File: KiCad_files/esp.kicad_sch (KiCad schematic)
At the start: 0 parts

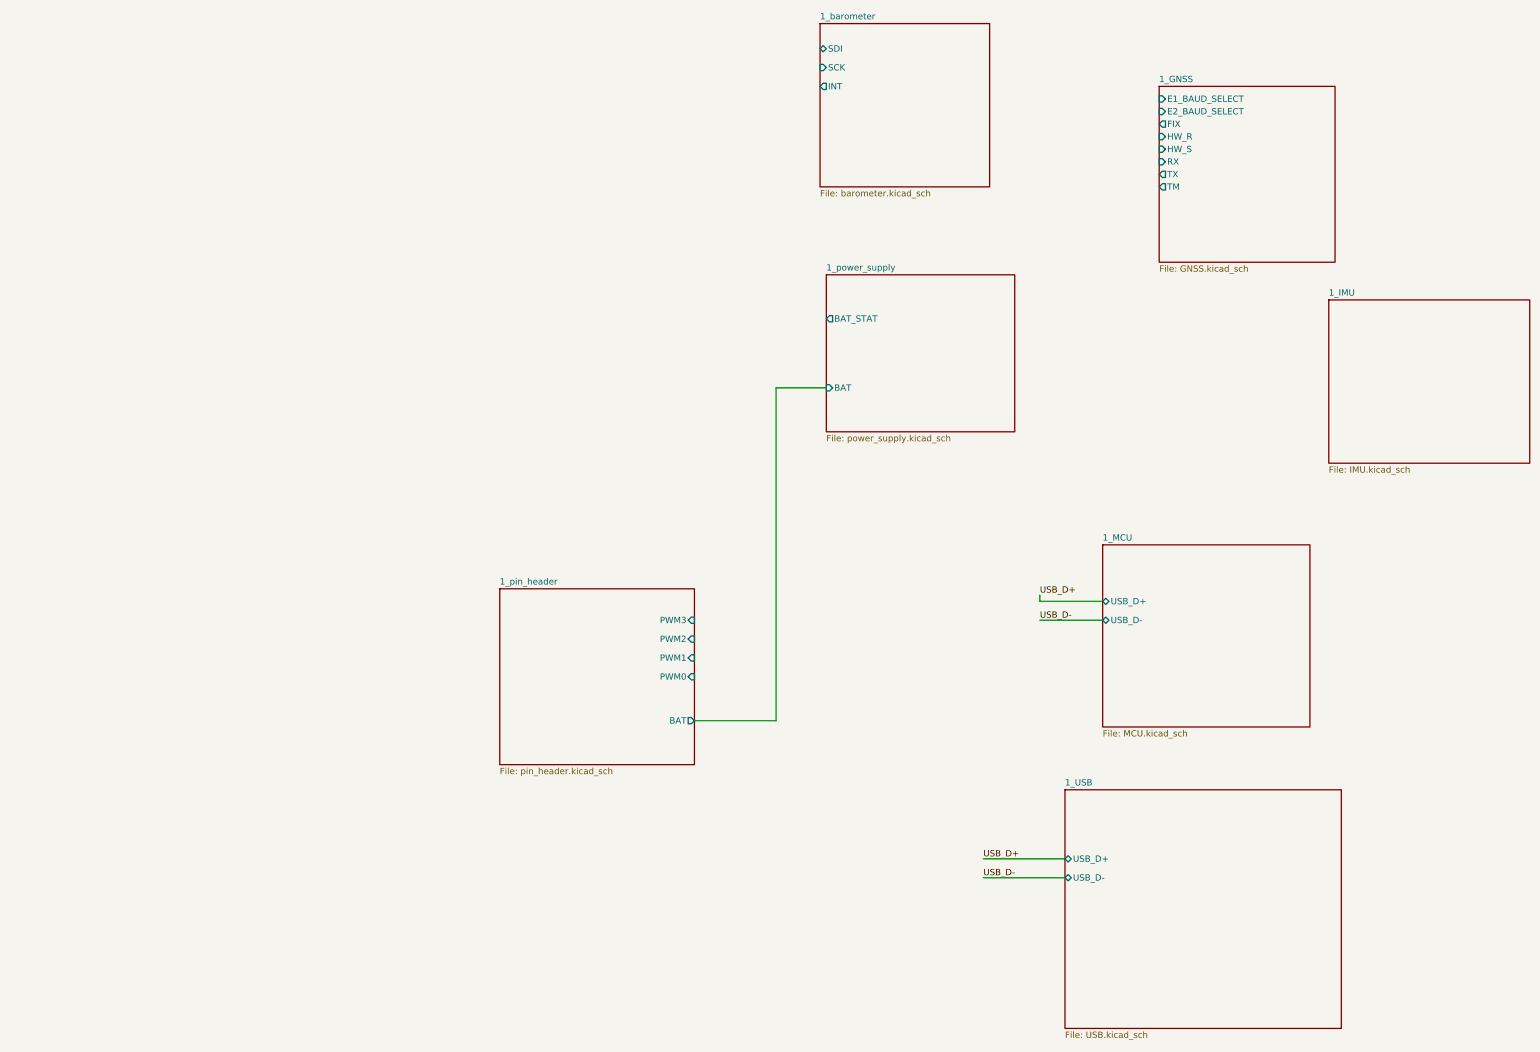
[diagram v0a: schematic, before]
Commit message: i2c
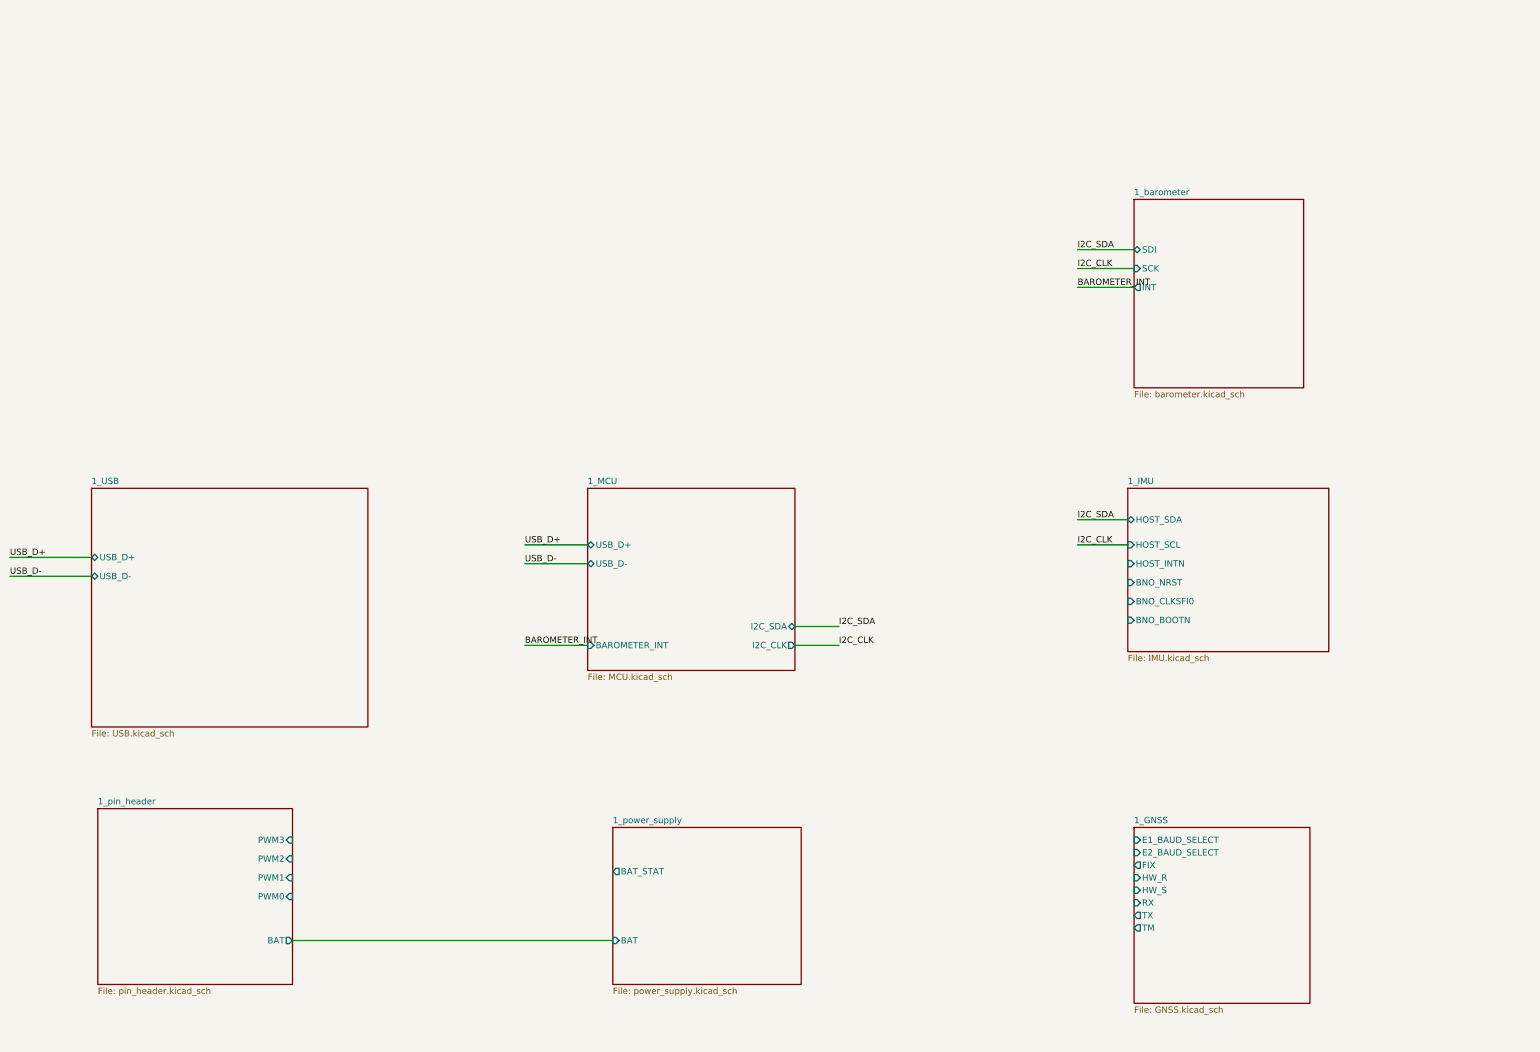
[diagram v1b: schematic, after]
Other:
- sheet 1_IMU ports: added BNO_BOOTN, BNO_CLKSFI0, BNO_NRST, HOST_INTN, HOST_SCL, HOST_SDA; removed none
- sheet 1_MCU ports: added BAROMETER_INT, I2C_CLK, I2C_SDA; removed none
